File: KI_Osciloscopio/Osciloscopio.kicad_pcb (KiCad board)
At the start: 2 copper layers, 98.8 x 73 mm, 37 parts, among them CN1 Conector IZQ, CN2 Conector DER, J1 VIN, J2 Conn_Coaxial, J3 DISPLAY, J4 USB_B, U1 MCP6004, U2 74HC4051, U4 LM1117-3.3, U5 M95128

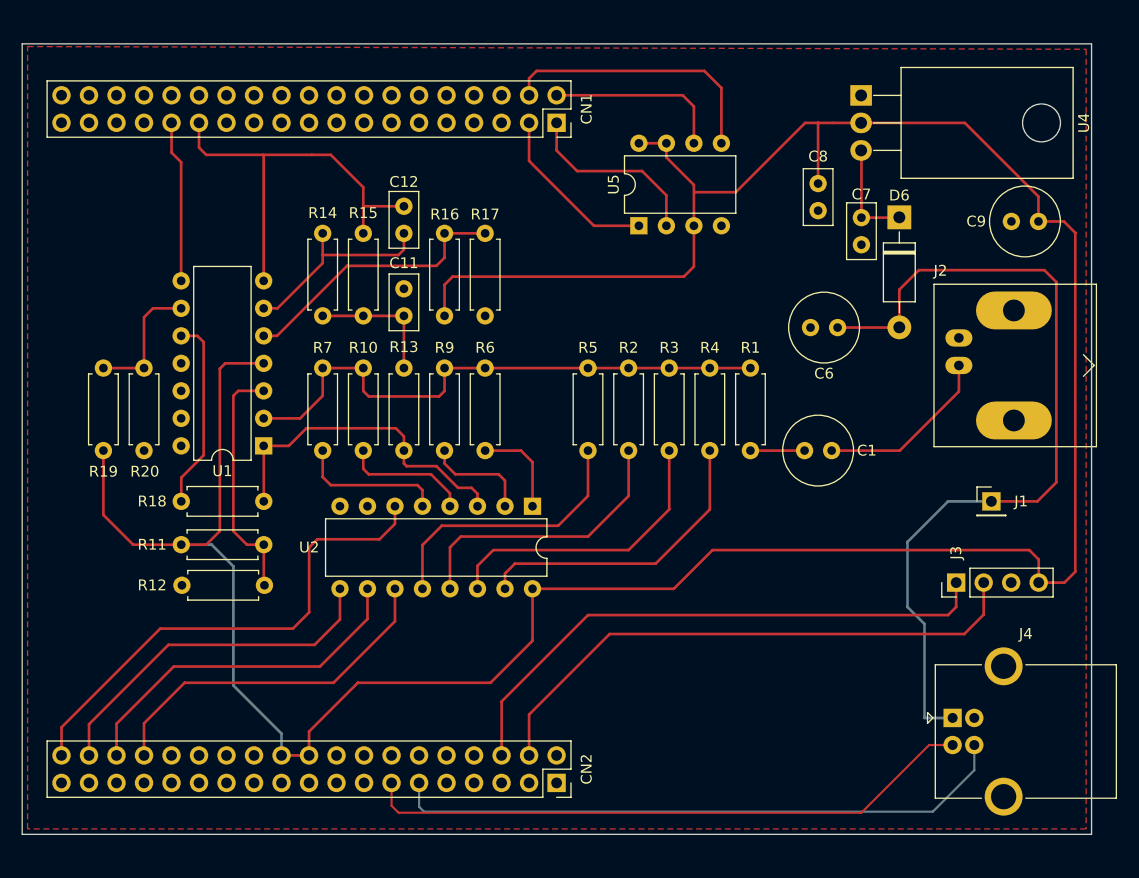
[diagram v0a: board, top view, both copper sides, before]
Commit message: Plaquita
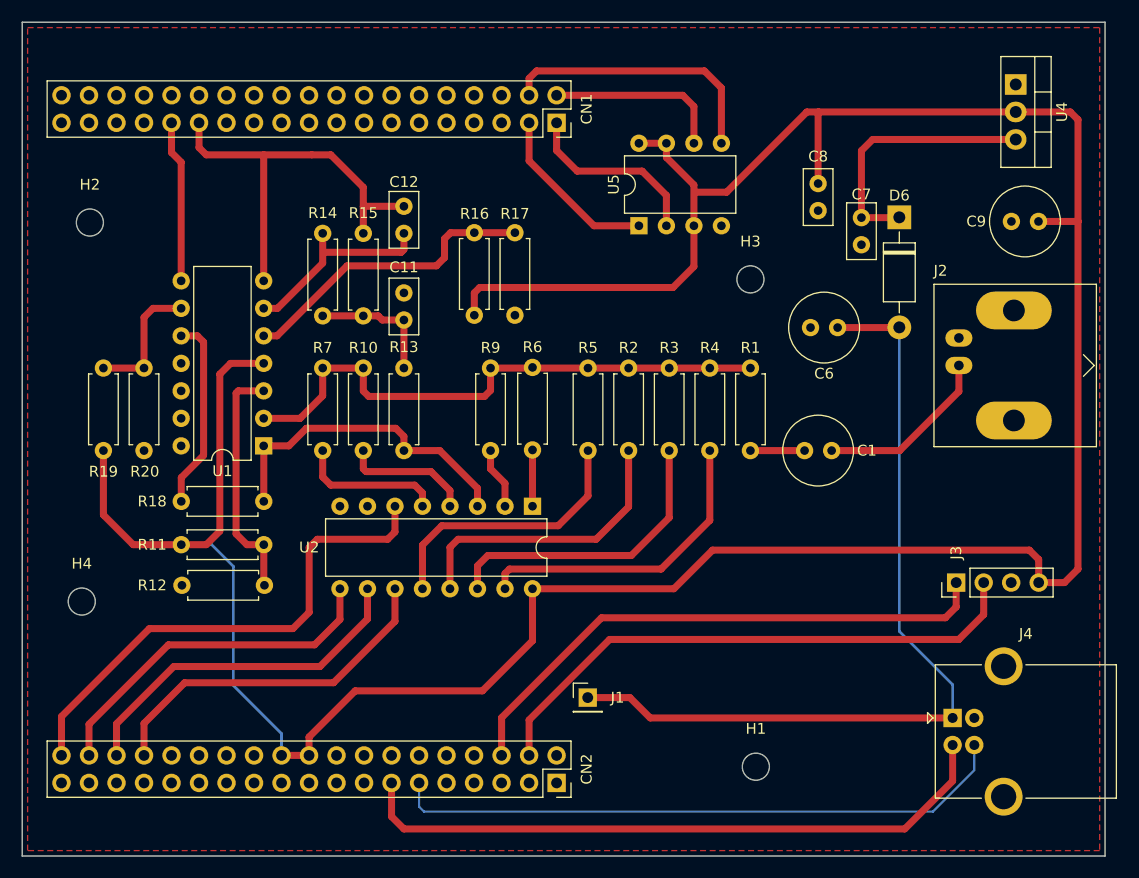
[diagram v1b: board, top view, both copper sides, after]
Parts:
- added H1: MountingHole, MountingHole:MountingHole_2.5mm, F.Cu at (97.2, 105.2)
- added H2: MountingHole, MountingHole:MountingHole_2.5mm, F.Cu at (35.8, 55.0)
- added H3: MountingHole, MountingHole:MountingHole_2.5mm, F.Cu at (96.8, 60.2)
- added H4: MountingHole, MountingHole:MountingHole_2.5mm, F.Cu at (35.0, 90.0)
- U4: footprint Package_TO_SOT_THT:TO-220-3_Horizontal_TabDown -> Package_TO_SOT_THT:TO-220-3_Vertical
- moved J1 41.4 mm to (81.7, 98.9)
- moved U4 14.3 mm to (121.2, 42.2)
- moved R6 4.38 mm to (76.6, 76.0)
- moved R9 4.25 mm to (72.8, 76.1)
- moved R16 2.75 mm to (71.2, 55.9)
- moved R17 2.75 mm to (75.0, 55.9)
- moved C11 0.38 mm to (64.8, 61.5)
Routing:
- net Net-(C7-Pad1): track 9.73 -> 24.4 mm
- net 3.3V: track 272.5 -> 279.3 mm
- net Net-(R9-Pad1): track 9.80 -> 5.69 mm
- net /D-: track 56.8 -> 60.6 mm
- net Net-(R6-Pad1): track 8.89 -> 5.20 mm
- net Net-(R16-Pad1): track 25.7 -> 28.2 mm
- net D0: track 46.3 -> 47.3 mm
- net /SDA: track 52.8 -> 51.9 mm
- net /VIN: track 78.9 -> 78.3 mm
- net Net-(R2-Pad2): track 26.7 -> 27.3 mm
- net Net-(R4-Pad1): track 28.4 -> 29.0 mm
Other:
- board size 98.8 x 73 mm -> 100 x 77 mm
